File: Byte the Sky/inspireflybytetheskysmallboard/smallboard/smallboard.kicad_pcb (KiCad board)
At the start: 2 copper layers, 23.3 x 21.5 mm, 15 parts, among them IC1 N34TS04MT3ETG, J1 Conn_01x07_Pin, U2 LSM6DSV, U4 LIS2MDLTR

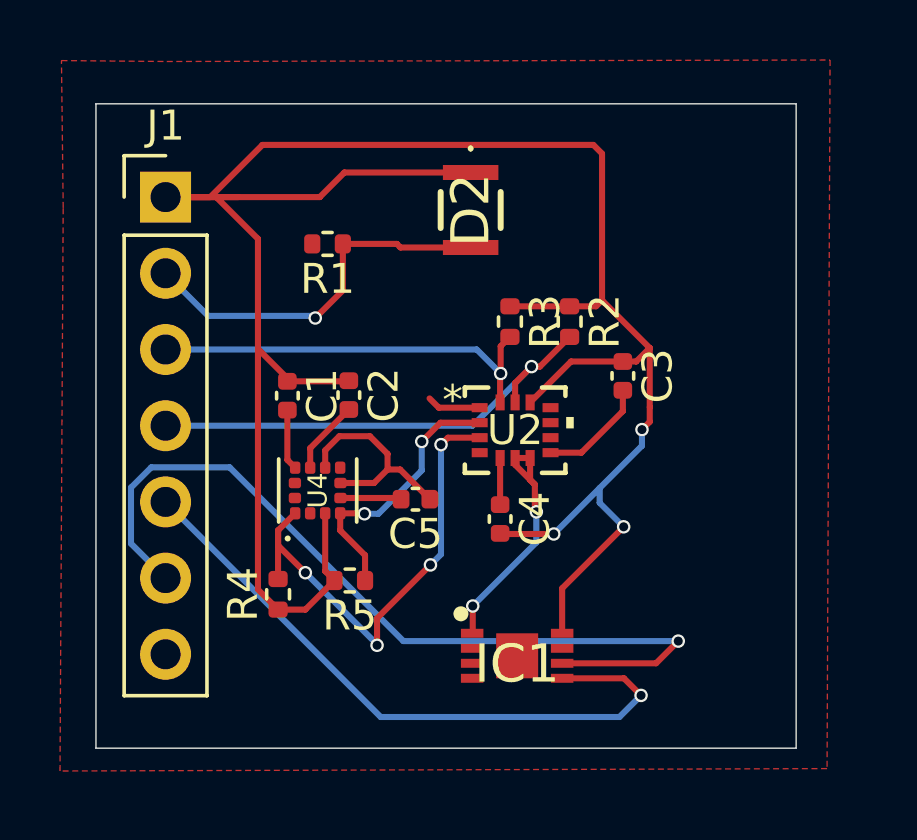
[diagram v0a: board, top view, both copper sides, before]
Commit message: Add files via upload
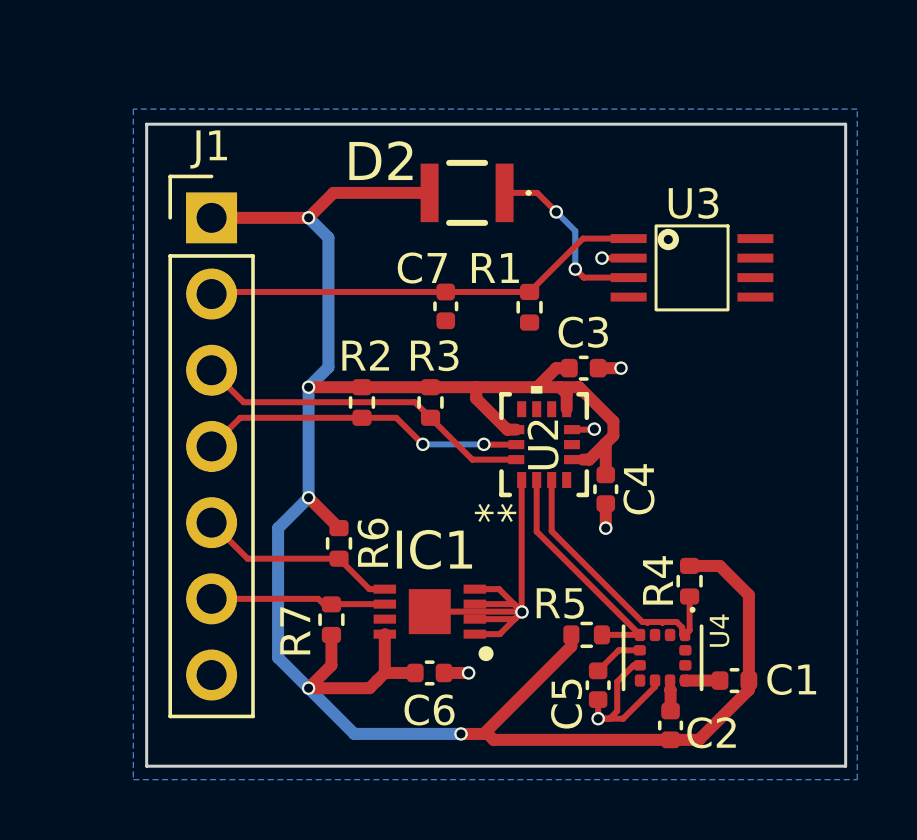
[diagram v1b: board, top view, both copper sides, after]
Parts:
- added C6: C, Capacitor_SMD:C_0402_1005Metric, F.Cu at (102.3, 75.7)
- added C7: 100nF, Capacitor_SMD:C_0402_1005Metric, F.Cu at (102.9, 63.5)
- added R6: 10k, Resistor_SMD:R_0402_1005Metric, F.Cu at (99.3, 71.4)
- added R7: 10k, Resistor_SMD:R_0402_1005Metric, F.Cu at (99.1, 73.9)
- added U3: OPA381, OPA381:MSOP08, F.Cu at (111.1, 62.2)
- D2: footprint VEMD:VEMD8083 -> footprints:VEMD8083
- IC1: footprint N34:SON50P300X200X80-9N -> footprints:SON50P300X200X80-9N
- U4: footprint LIS2MDLTR:PQFN50P200X200X70-12N -> footprints:PQFN50P200X200X70-12N
- moved C1 17.7 mm to (112.5, 75.9), turned to 180 degrees
- moved C2 15.4 mm to (110.4, 77.4), turned to 90 degrees
- moved R4 13.7 mm to (111.0, 72.6), turned to -90 degrees
- moved U4 12.8 mm to (110.1, 75.2), turned to -90 degrees
- moved C5 8.69 mm to (108.0, 76.1), turned to 90 degrees
- moved R5 8.10 mm to (107.6, 74.4)
- moved R2 7.43 mm to (100.1, 66.7)
- moved R1 7.06 mm to (105.7, 63.5), turned to 90 degrees
- moved R3 3.78 mm to (102.4, 66.7)
- moved C4 3.66 mm to (108.2, 69.6), turned to 90 degrees
- moved IC1 3.26 mm to (102.3, 73.6), turned to 180 degrees
- moved J1 1.68 mm to (95.1, 60.5)
- moved C3 1.33 mm to (107.5, 65.5), turned to 0 degrees
- moved U2 1.08 mm to (106.2, 68.1), turned to 90 degrees
- moved D2 0.58 mm to (103.6, 59.7), turned to 0 degrees
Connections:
- C3 pad 2: Net-(U2-VDD) -> GND
- C4 pad 1: Net-(U2-VDD_IO) -> GND
- D2 pad 1: +3.3V -> Net-(D2-K)
- D2 pad 2: ADC_0 -> +3.3V
- IC1 pad 9: unconnected-(IC1-EP-Pad9) -> GND
- R1 pad 1: ADC_0 -> Net-(D2-K)
- R1 pad 2: GND -> ADC_0
- U2 pad 5: Net-(U2-VDD_IO) -> +3.3V
- U2 pad 8: Net-(U2-VDD) -> +3.3V
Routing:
- net GPIO_17: track 28.6 -> 5.85 mm, vias 1 -> 0
- net GPIO_16: track 22.0 -> 6.69 mm, vias 1 -> 0
- net Net-(U2-SCX): track 16.6 -> 9.12 mm, vias 4 -> 0
- net GND: track 17.5 -> 24.5 mm, vias 2 -> 7
- net Net-(D2-K): track 0.00 -> 6.05 mm, vias 0 -> 2
- net GPIO_15: track 16.1 -> 10.9 mm, vias 1 -> 2
- net +3.3V: track 81.5 -> 77.6 mm, vias 3 -> 5
- net Net-(U2-VDD): track 3.68 -> 0.00 mm
- net GPIO_14: track 13.8 -> 11.4 mm, vias 1 -> 0
- net ADC_0: track 12.8 -> 14.7 mm, vias 1 -> 0
- net Net-(U4-VDD): track 2.47 -> 0.73 mm
- net Net-(U2-VDD_IO): track 1.65 -> 0.00 mm
- net Net-(U2-SDX): track 9.06 -> 7.86 mm, vias 2 -> 0
- net Net-(U4-VDD_IO): track 2.03 -> 1.16 mm
- added copper zone on B.Cu, net GND
- removed copper zone on F.Cu, net GND
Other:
- board size 23.3 x 21.5 mm -> 23.3 x 21.4 mm
